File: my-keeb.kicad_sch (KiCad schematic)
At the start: 183 parts, among them SW10 SW_Push, SW11 SW_Push, SW12 SW_Push, SW13 SW_Push, SW14 SW_Push, SW16 SW_Push, SW17 SW_Push, SW18 SW_Push, SW19 SW_Push, SW2 SW_Push, SW20 SW_Push, SW21 SW_Push, SW22 SW_Push, SW23 SW_Push, SW24 SW_Push, SW25 SW_Push, SW26 SW_Push, SW27 SW_Push, SW29 SW_Push, SW3 SW_Push, SW30 SW_Push, SW31 SW_Push, SW32 SW_Push, SW33 SW_Push, SW34 SW_Push, SW35 SW_Push, SW36 SW_Push, SW37 SW_Push, SW38 SW_Push, SW39 SW_Push, SW4 SW_Push, SW40 SW_Push, SW41 SW_Push, SW42 SW_Push, SW43 SW_Push, SW44 SW_Push, SW45 SW_Push, SW46 SW_Push, SW47 SW_Push, SW48 SW_Push, SW49 SW_Push, SW5 SW_Push, SW50 SW_Push, SW51 SW_Push, SW52 SW_Push, SW53 SW_Push, SW54 SW_Push, SW55 SW_Push, SW57 SW_Push, SW58 SW_Push, SW6 SW_Push, SW60 SW_Push, SW61 SW_Push, SW62 SW_Push, SW63 SW_Push, SW64 SW_Push, SW65 SW_Push, SW66 SW_Push, SW67 SW_Push, SW68 SW_Push, SW69 SW_Push, SW7 SW_Push, SW71 SW_Push, SW72 SW_Push, SW73 SW_Push, SW74 SW_Push, SW75 SW_Push, SW77 SW_Push, SW79 SW_Push, SW8 SW_Push, SW80 SW_Push, SW81 SW_Push, SW82 SW_Push, SW84 SW_Push, SW85 SW_Push, SW86 SW_Push, SW87 SW_Push, SW88 SW_Push, SW89 SW_Push, SW9 SW_Push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

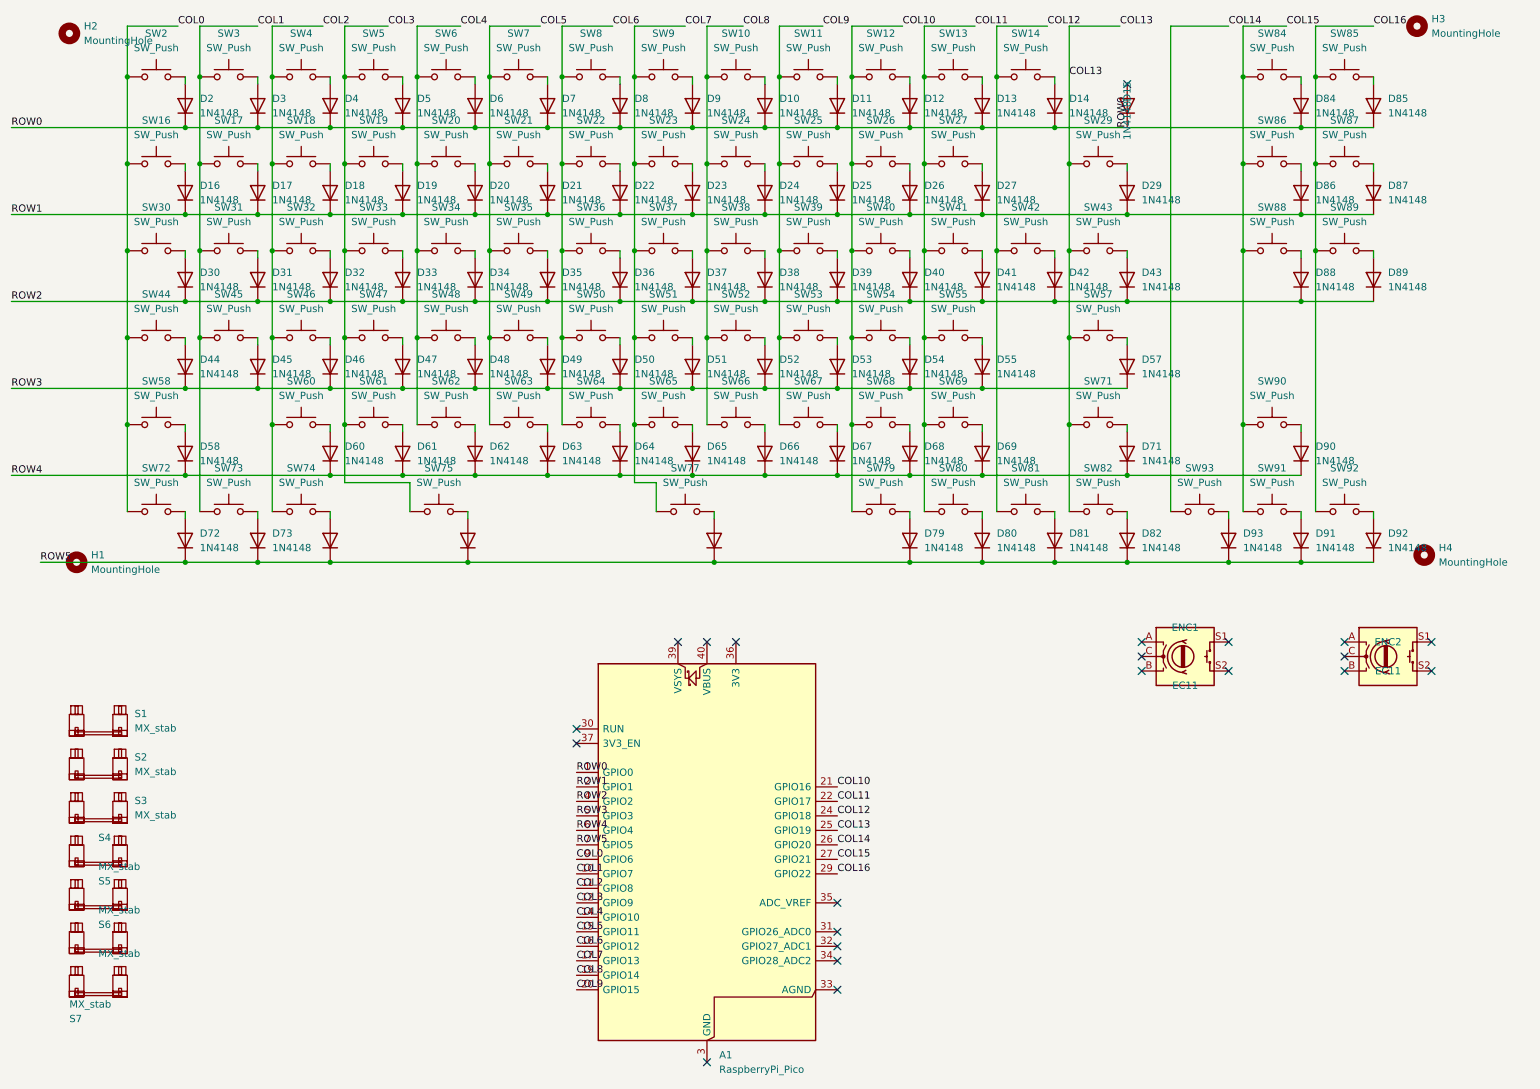
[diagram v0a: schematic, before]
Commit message: Add files via upload
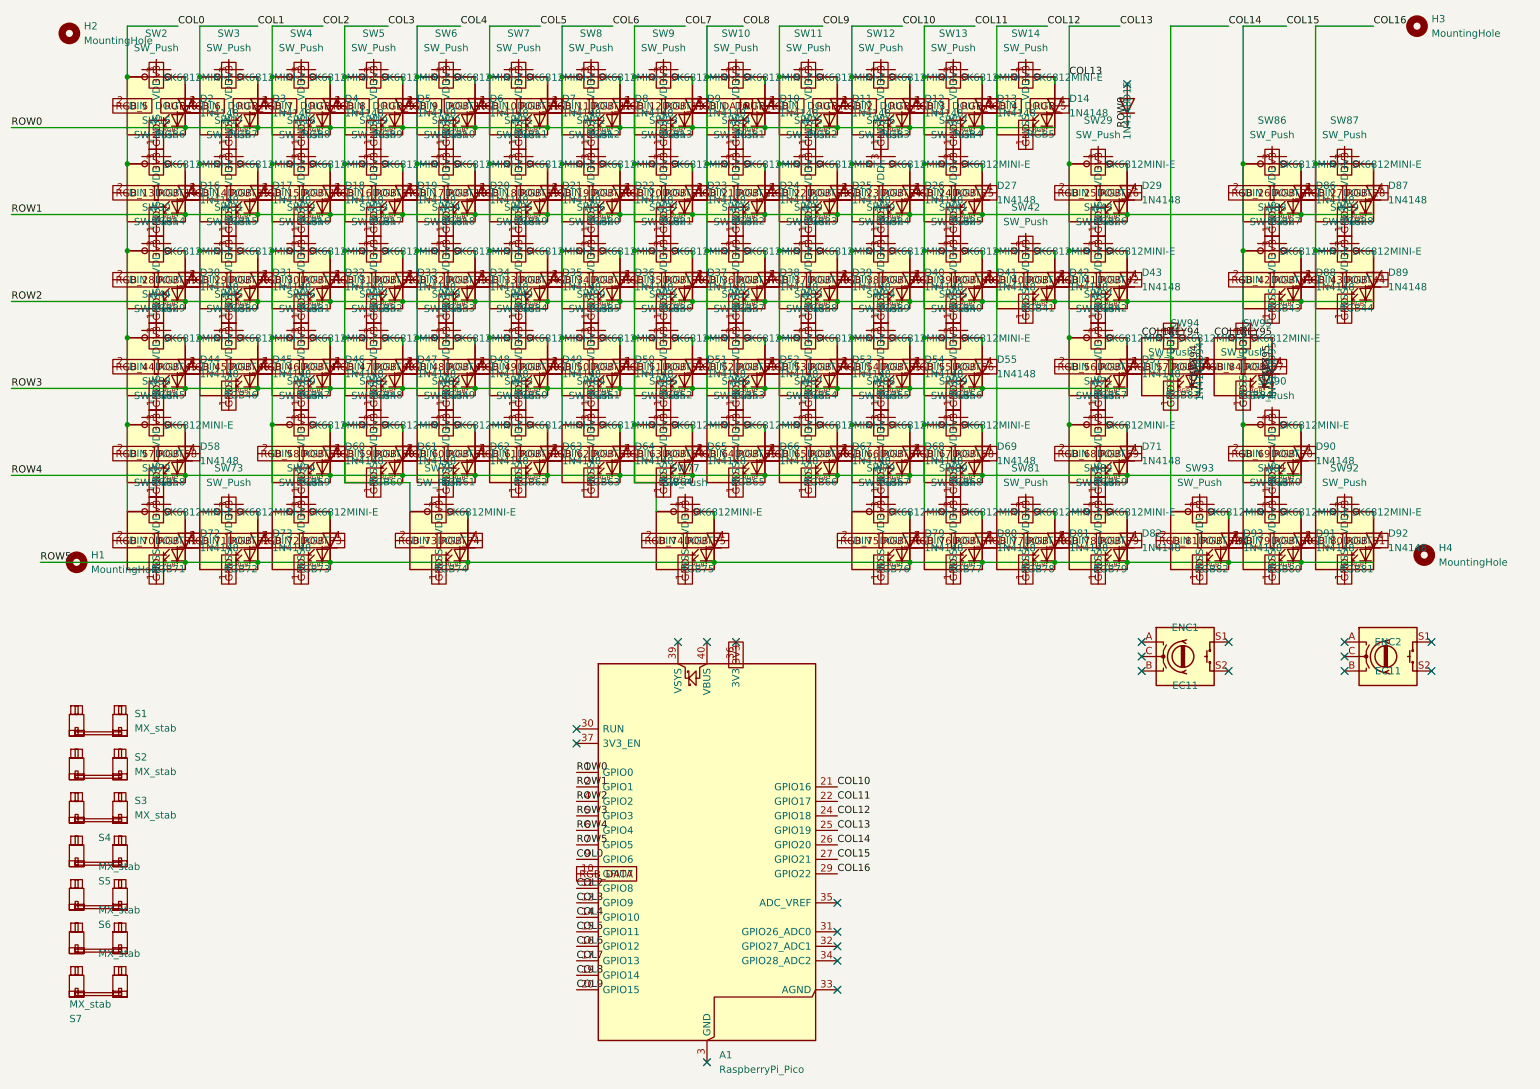
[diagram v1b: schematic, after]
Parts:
- removed D84, D85: 1N4148, Diode_THT:D_DO-35_SOD27_P7.62mm_Horizontal, symbol Diode:1N4148
- removed SW84, SW85: SW_Push, PCM_marbastlib-mx:SW_MX_1u, symbol Switch:SW_Push
- added D94, D95: 1N4148, Diode_THT:D_DO-35_SOD27_P7.62mm_Horizontal, symbol Diode:1N4148
- added RGB1, RGB10, RGB11, RGB12, RGB13, RGB14, RGB15, RGB16, RGB17, RGB18, RGB19, RGB2, RGB20, RGB21, RGB22, RGB23, RGB24, RGB25, RGB26, RGB27, RGB28, RGB29, RGB3, RGB30, RGB31, RGB32, RGB33, RGB35, RGB36, RGB37, RGB38, RGB39, RGB4, RGB40, RGB41, RGB42, RGB43, RGB44, RGB45, RGB46, RGB47, RGB48, RGB49, RGB5, RGB50, RGB51, RGB52, RGB53, RGB54, RGB55, RGB56, RGB57, RGB58, RGB59, RGB6, RGB60, RGB61, RGB62, RGB63, RGB64, RGB65, RGB66, RGB67, RGB68, RGB69, RGB7, RGB70, RGB71, RGB72, RGB73, RGB74, RGB75, RGB76, RGB77, RGB78, RGB79, RGB8, RGB80, RGB81, RGB82, RGB83, RGB84, RGB9: SK6812MINI-E, LED_SMD:LED_SK6812MINI-E_3.2x2.8mm_P1.5mm_ReverseMount, symbol LED:SK6812MINI-E
- added RGB34: SK6812MINI-E, my-keeb:LED_SK6812MINI-E_3.2x2.8mm_P1.5mm_ReverseMount, symbol LED:SK6812MINI-E
- added SW94, SW95: SW_Push, PCM_marbastlib-mx:SW_MX_1u, symbol Switch:SW_Push
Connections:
- net COL14 is gone; now on net 3V3: A1.26 (GPIO20), SW93.1
- net COL15 is gone; now on net 3V3: A1.27 (GPIO21), SW86.1, SW88.1, SW90.1, SW91.1
- net ROW3: now also D94.1 (K), D95.1 (K)
- net 3V3: now reaches A1.36 (3V3)
- net 3V3: now also RGB1.1 (VSS), RGB1.3 (VDD), RGB10.1 (VSS), RGB10.3 (VDD), RGB11.1 (VSS), RGB11.3 (VDD), RGB12.1 (VSS), RGB12.3 (VDD), RGB13.1 (VSS), RGB13.3 (VDD), RGB14.1 (VSS), RGB14.3 (VDD), RGB15.1 (VSS), RGB15.3 (VDD), RGB16.1 (VSS), RGB16.3 (VDD), RGB17.1 (VSS), RGB17.3 (VDD), RGB18.1 (VSS), RGB18.3 (VDD), RGB19.1 (VSS), RGB19.3 (VDD), RGB2.1 (VSS), RGB2.3 (VDD), RGB20.1 (VSS), RGB20.3 (VDD), RGB21.1 (VSS), RGB21.3 (VDD), RGB22.1 (VSS), RGB22.3 (VDD), RGB23.1 (VSS), RGB23.3 (VDD), RGB24.1 (VSS), RGB24.3 (VDD), RGB25.1 (VSS), RGB25.3 (VDD), RGB26.1 (VSS), RGB26.3 (VDD), RGB27.1 (VSS), RGB27.3 (VDD), RGB28.1 (VSS), RGB28.3 (VDD), RGB29.1 (VSS), RGB29.3 (VDD), RGB3.1 (VSS), RGB3.3 (VDD), RGB30.1 (VSS), RGB30.3 (VDD), RGB31.1 (VSS), RGB31.3 (VDD), RGB32.1 (VSS), RGB32.3 (VDD), RGB33.1 (VSS), RGB33.3 (VDD), RGB34.1 (VSS), RGB34.3 (VDD), RGB35.1 (VSS), RGB35.3 (VDD), RGB36.1 (VSS), RGB36.3 (VDD), RGB37.1 (VSS), RGB37.3 (VDD), RGB38.1 (VSS), RGB38.3 (VDD), RGB39.1 (VSS), RGB39.3 (VDD), RGB4.1 (VSS), RGB4.3 (VDD), RGB40.1 (VSS), RGB40.3 (VDD), RGB41.1 (VSS), RGB41.3 (VDD), RGB42.1 (VSS), RGB42.3 (VDD), RGB43.1 (VSS), RGB43.3 (VDD), RGB44.1 (VSS), RGB44.3 (VDD), RGB45.1 (VSS), RGB45.3 (VDD), RGB46.1 (VSS), RGB46.3 (VDD), RGB47.1 (VSS), RGB47.3 (VDD), RGB48.1 (VSS), RGB48.3 (VDD), RGB49.1 (VSS), RGB49.3 (VDD), RGB5.1 (VSS), RGB5.3 (VDD), RGB50.1 (VSS), RGB50.3 (VDD), RGB51.1 (VSS), RGB51.3 (VDD), RGB52.1 (VSS), RGB52.3 (VDD), RGB53.1 (VSS), RGB53.3 (VDD), RGB54.1 (VSS), RGB54.3 (VDD), RGB55.1 (VSS), RGB55.3 (VDD), RGB56.1 (VSS), RGB56.3 (VDD), RGB57.1 (VSS), RGB57.3 (VDD), RGB58.1 (VSS), RGB58.3 (VDD), RGB59.1 (VSS), RGB59.3 (VDD), RGB6.1 (VSS), RGB6.3 (VDD), RGB60.1 (VSS), RGB60.3 (VDD), RGB61.1 (VSS), RGB61.3 (VDD), RGB62.1 (VSS), RGB62.3 (VDD), RGB63.1 (VSS), RGB63.3 (VDD), RGB64.1 (VSS), RGB64.3 (VDD), RGB65.1 (VSS), RGB65.3 (VDD), RGB66.1 (VSS), RGB66.3 (VDD), RGB67.1 (VSS), RGB67.3 (VDD), RGB68.1 (VSS), RGB68.3 (VDD), RGB69.1 (VSS), RGB69.3 (VDD), RGB7.1 (VSS), RGB7.3 (VDD), RGB70.1 (VSS), RGB70.3 (VDD), RGB71.1 (VSS), RGB71.3 (VDD), RGB72.1 (VSS), RGB72.3 (VDD), RGB73.1 (VSS), RGB73.3 (VDD), RGB74.1 (VSS), RGB74.3 (VDD), RGB75.1 (VSS), RGB75.3 (VDD), RGB76.1 (VSS), RGB76.3 (VDD), RGB77.1 (VSS), RGB77.3 (VDD), RGB78.1 (VSS), RGB78.3 (VDD), RGB79.1 (VSS), RGB79.3 (VDD), RGB8.1 (VSS), RGB8.3 (VDD), RGB80.1 (VSS), RGB80.3 (VDD), RGB81.1 (VSS), RGB81.3 (VDD), RGB82.1 (VSS), RGB82.3 (VDD), RGB83.1 (VSS), RGB83.3 (VDD), RGB84.1 (VSS), RGB84.3 (VDD), RGB9.1 (VSS), RGB9.3 (VDD), SW94.1, SW95.1
- net COL1 renamed RGB_14
- net RGB_14: now also RGB14.4 (DOUT), RGB15.2 (DIN), RGB29.4 (DOUT), RGB30.2 (DIN), RGB45.4 (DOUT), RGB46.2 (DIN), RGB58.4 (DOUT), RGB59.2 (DIN), RGB6.4 (DOUT), RGB7.2 (DIN); no longer A1.10 (GPIO7)
- net COL10 renamed RGB_2
- net RGB_2: now also RGB2.4 (DOUT), RGB23.4 (DOUT), RGB24.2 (DIN), RGB3.2 (DIN), RGB38.4 (DOUT), RGB39.2 (DIN), RGB54.4 (DOUT), RGB55.2 (DIN), RGB66.4 (DOUT), RGB67.2 (DIN)
- net COL11 renamed RGB_24
- net RGB_24: now also RGB24.4 (DOUT), RGB25.2 (DIN), RGB3.4 (DOUT), RGB39.4 (DOUT), RGB4.2 (DIN), RGB40.2 (DIN), RGB55.4 (DOUT), RGB56.2 (DIN), RGB67.4 (DOUT), RGB68.2 (DIN)
- net COL12 renamed RGB_25
- net RGB_25: now also RGB25.4 (DOUT), RGB26.2 (DIN), RGB4.4 (DOUT), RGB40.4 (DOUT), RGB41.2 (DIN), RGB5.2 (DIN), RGB56.4 (DOUT), RGB57.2 (DIN), RGB68.4 (DOUT), RGB69.2 (DIN)
- net COL13 renamed RGB_41
- net RGB_41: now also RGB41.4 (DOUT), RGB42.2 (DIN), RGB5.4 (DOUT), RGB6.2 (DIN)
- net COL16 renamed RGB_27
- net RGB_27: now also RGB27.4 (DOUT), RGB28.2 (DIN), RGB43.4 (DOUT), RGB44.2 (DIN), RGB70.4 (DOUT), RGB71.2 (DIN)
- net COL2 renamed RGB_15
- net RGB_15: now also RGB15.4 (DOUT), RGB16.2 (DIN), RGB30.4 (DOUT), RGB31.2 (DIN), RGB46.4 (DOUT), RGB47.2 (DIN), RGB7.4 (DOUT), RGB8.2 (DIN)
- net COL3 renamed RGB_16
- net RGB_16: now also RGB16.4 (DOUT), RGB17.2 (DIN), RGB31.4 (DOUT), RGB32.2 (DIN), RGB47.4 (DOUT), RGB48.2 (DIN), RGB59.4 (DOUT), RGB60.2 (DIN), RGB8.4 (DOUT), RGB9.2 (DIN)
- net COL4 renamed RGB_17
- net RGB_17: now also RGB10.2 (DIN), RGB17.4 (DOUT), RGB18.2 (DIN), RGB32.4 (DOUT), RGB33.2 (DIN), RGB48.4 (DOUT), RGB49.2 (DIN), RGB9.4 (DOUT)
- net COL5 renamed RGB_10
- net RGB_10: now also RGB10.4 (DOUT), RGB11.2 (DIN), RGB18.4 (DOUT), RGB19.2 (DIN), RGB33.4 (DOUT), RGB34.2 (DIN), RGB49.4 (DOUT), RGB50.2 (DIN)
- net COL6 renamed RGB_11
- net RGB_11: now also RGB11.4 (DOUT), RGB12.2 (DIN), RGB19.4 (DOUT), RGB20.2 (DIN), RGB34.4 (DOUT), RGB35.2 (DIN), RGB50.4 (DOUT), RGB51.2 (DIN)
- net COL7 renamed RGB_12
- net RGB_12: now also RGB12.4 (DOUT), RGB13.2 (DIN), RGB20.4 (DOUT), RGB21.2 (DIN), RGB35.4 (DOUT), RGB36.2 (DIN), RGB51.4 (DOUT), RGB52.2 (DIN), RGB63.4 (DOUT), RGB64.2 (DIN)
- net COL8 renamed RGB_13
- net RGB_13: now also RGB13.4 (DOUT), RGB14.2 (DIN), RGB21.4 (DOUT), RGB22.2 (DIN), RGB36.4 (DOUT), RGB37.2 (DIN), RGB52.4 (DOUT), RGB53.2 (DIN)
- net COL9 renamed RGB_1
- net RGB_1: now also RGB1.4 (DOUT), RGB2.2 (DIN), RGB22.4 (DOUT), RGB23.2 (DIN), RGB37.4 (DOUT), RGB38.2 (DIN), RGB53.4 (DOUT), RGB54.2 (DIN)
- new net KEY94: D94.2 (A), SW94.2
- new net KEY95: D95.2 (A), SW95.2
- new net RGB_26: RGB26.4 (DOUT), RGB27.2 (DIN)
- new net RGB_28: RGB28.4 (DOUT), RGB29.2 (DIN)
- new net RGB_42: RGB42.4 (DOUT), RGB43.2 (DIN)
- new net RGB_44: RGB44.4 (DOUT), RGB45.2 (DIN)
- new net RGB_57: RGB57.4 (DOUT), RGB58.2 (DIN), RGB83.2 (DIN), RGB84.4 (DOUT)
- new net RGB_60: RGB60.4 (DOUT), RGB61.2 (DIN)
- new net RGB_61: RGB61.4 (DOUT), RGB62.2 (DIN)
- new net RGB_62: RGB62.4 (DOUT), RGB63.2 (DIN)
- new net RGB_64: RGB64.4 (DOUT), RGB65.2 (DIN)
- new net RGB_65: RGB65.4 (DOUT), RGB66.2 (DIN)
- new net RGB_69: RGB69.4 (DOUT), RGB70.2 (DIN)
- new net RGB_71: RGB71.4 (DOUT), RGB72.2 (DIN)
- new net RGB_72: RGB72.4 (DOUT), RGB73.2 (DIN)
- new net RGB_73: RGB73.4 (DOUT), RGB74.2 (DIN)
- new net RGB_74: RGB74.4 (DOUT), RGB75.2 (DIN)
- new net RGB_75: RGB75.4 (DOUT), RGB76.2 (DIN)
- new net RGB_76: RGB76.4 (DOUT), RGB77.2 (DIN)
- new net RGB_77: RGB77.4 (DOUT), RGB78.2 (DIN)
- new net RGB_78: RGB78.4 (DOUT), RGB79.2 (DIN)
- new net RGB_79: RGB79.4 (DOUT), RGB80.2 (DIN)
- new net RGB_80: RGB80.4 (DOUT), RGB81.2 (DIN)
- new net RGB_81: RGB81.4 (DOUT), RGB82.2 (DIN)
- new net RGB_82: RGB82.4 (DOUT)
- new net RGB_84: RGB83.4 (DOUT), RGB84.2 (DIN)
- new net RGB_DATA: A1.10 (GPIO7), RGB1.2 (DIN)
- no-connect marks 22 -> 23
